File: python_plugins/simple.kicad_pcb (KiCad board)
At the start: 2 copper layers, 43 x 11 mm, 3 parts, among them P101 CONN_01X02, P102 CONN_01X02, P103 CONN_01X02

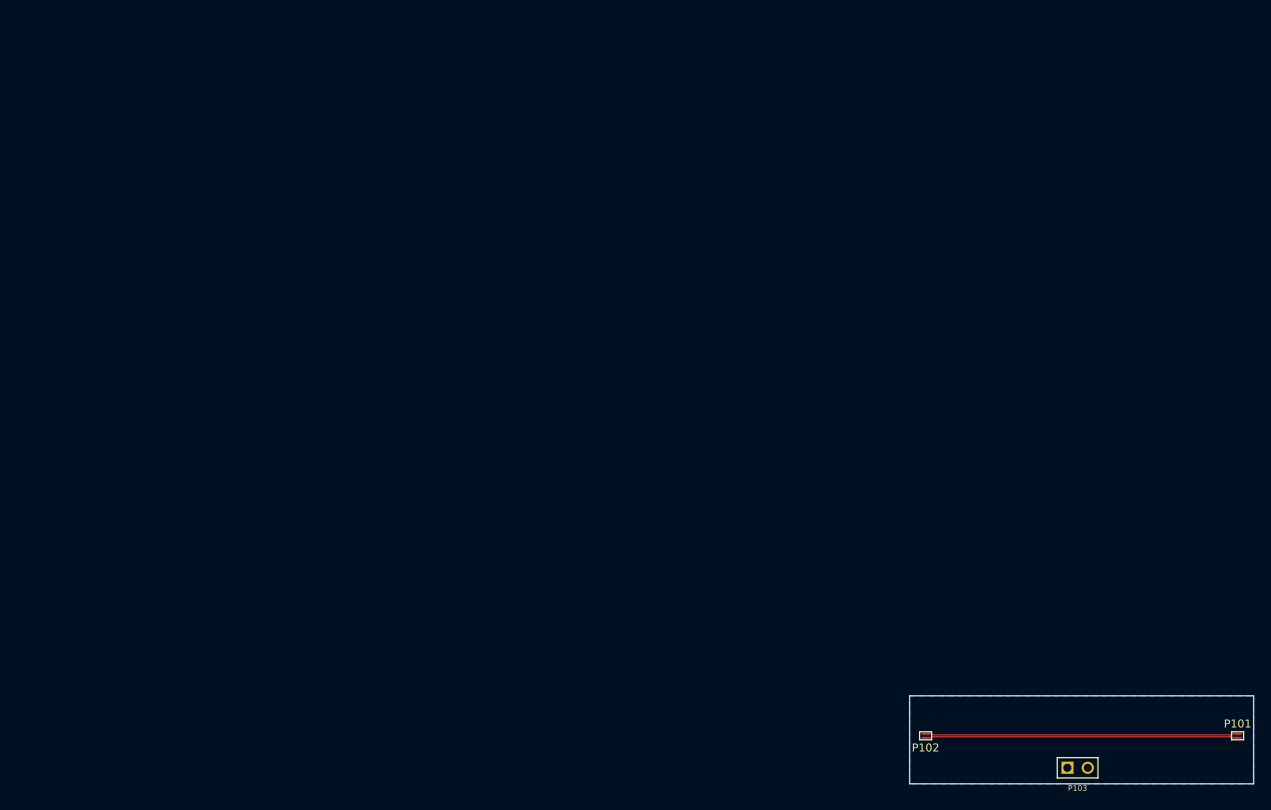
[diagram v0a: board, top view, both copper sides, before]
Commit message: wip
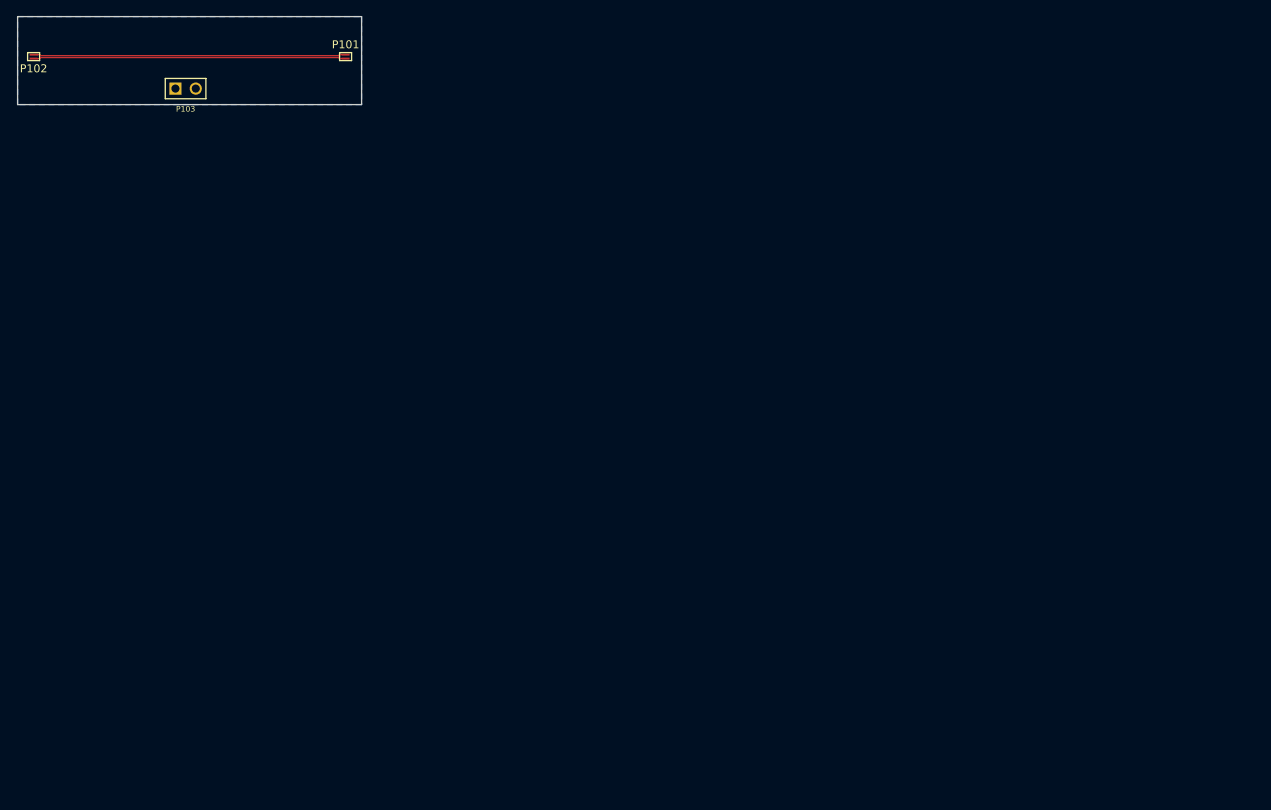
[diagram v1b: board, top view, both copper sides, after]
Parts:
- moved P101 140.1 mm to (55.5, 20.1)
- moved P102 140.1 mm to (16.5, 20.1)
- moved P103 140.1 mm to (35.5, 24.1)
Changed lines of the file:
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@@
   (general
     (links 3)
-    (no_connects 2)
+    (no_connects 0)
     (area 122.891667 99.924999 172.108334 112.316)
     (thickness 1.6)
@@
   )
   (module Connectors_254mm:pin_array_2x1 (layer F.Cu)
-    (at 147 109)
+    (at 35.5 24.1)
     (descr "Connecteurs 2 pins")
     (tags "CONN DEV")
@@
   )
   (module test:TEST_01x02_05mm (layer F.Cu)
-    (at 167 105 180)
+    (at 55.5 20.1 180)
     (attr smd)
     (fp_text reference P101 (at 0 1.5 180) (layer F.SilkS)
@@
   )
   (module test:TEST_01x02_05mm (layer F.Cu)
-    (at 128 105)
+    (at 16.5 20.1)
     (attr smd)
     (fp_text reference P102 (at 0 1.5) (layer F.SilkS)
@@
       (net 2 /HS_P))
   )
-  (gr_line (start 126 111) (end 169 111) (layer Edge.Cuts) (width 0.15))
-  (gr_line (start 126 111) (end 126 100) (layer Edge.Cuts) (width 0.15))
-  (gr_line (start 169 100) (end 169 111) (layer Edge.Cuts) (width 0.15))
-  (gr_line (start 126 100) (end 169 100) (layer Edge.Cuts) (width 0.15))
-  (segment (start 128 105.25) (end 128.75 105.25) (width 0.12) (layer F.Cu) (net 2))
-  (segment (start 166.12 105.12) (end 166.25 105.25) (width 0.12) (layer F.Cu) (net 2))
-  (segment (start 128.75 105.25) (end 128.88 105.12) (width 0.12) (layer F.Cu) (net 2))
-  (segment (start 128.88 105.12) (end 166.12 105.12) (width 0.12) (layer F.Cu) (net 2))
-  (segment (start 166.25 105.25) (end 167 105.25) (width 0.12) (layer F.Cu) (net 2))
-  (segment (start 166.12 104.88) (end 166.25 104.75) (width 0.12) (layer F.Cu) (net 3))
-  (segment (start 166.25 104.75) (end 167 104.75) (width 0.12) (layer F.Cu) (net 3))
-  (segment (start 128 104.75) (end 128.75 104.75) (width 0.12) (layer F.Cu) (net 3))
-  (segment (start 128.75 104.75) (end 128.88 104.88) (width 0.12) (layer F.Cu) (net 3))
-  (segment (start 128.88 104.88) (end 166.12 104.88) (width 0.12) (layer F.Cu) (net 3))
+  (gr_line (start 14.5 26.1) (end 57.5 26.1) (layer Edge.Cuts) (width 0.15))
+  (gr_line (start 14.5 26.1) (end 14.5 15.1) (layer Edge.Cuts) (width 0.15))
+  (gr_line (start 57.5 15.1) (end 57.5 26.1) (layer Edge.Cuts) (width 0.15))
+  (gr_line (start 14.5 15.1) (end 57.5 15.1) (layer Edge.Cuts) (width 0.15))
+  (segment (start 16.5 20.35) (end 17.25 20.35) (width 0.12) (layer F.Cu) (net 2))
+  (segment (start 54.62 20.22) (end 54.75 20.35) (width 0.12) (layer F.Cu) (net 2))
+  (segment (start 17.25 20.35) (end 17.38 20.22) (width 0.12) (layer F.Cu) (net 2))
+  (segment (start 17.38 20.22) (end 54.62 20.22) (width 0.12) (layer F.Cu) (net 2))
+  (segment (start 54.75 20.35) (end 55.5 20.35) (width 0.12) (layer F.Cu) (net 2))
+  (segment (start 54.62 19.98) (end 54.75 19.85) (width 0.12) (layer F.Cu) (net 3))
+  (segment (start 54.75 19.85) (end 55.5 19.85) (width 0.12) (layer F.Cu) (net 3))
+  (segment (start 16.5 19.85) (end 17.25 19.85) (width 0.12) (layer F.Cu) (net 3))
+  (segment (start 17.25 19.85) (end 17.38 19.98) (width 0.12) (layer F.Cu) (net 3))
+  (segment (start 17.38 19.98) (end 54.62 19.98) (width 0.12) (layer F.Cu) (net 3))
   (zone (net 1) (net_name GND) (layer B.Cu) (hatch edge 0.508)
     (connect_pads yes (clearance 0.15))
@@
     (polygon
       (pts
-        (xy 126 100) (xy 169 100) (xy 169 111) (xy 126 111)
+        (xy 14.5 15.1) (xy 57.5 15.1) (xy 57.5 26.1) (xy 14.5 26.1)
       )
     )
